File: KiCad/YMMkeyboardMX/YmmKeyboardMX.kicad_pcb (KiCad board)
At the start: 2 copper layers, 259.1 x 139.7 mm, 123 parts, among them J3 RGB, SW10 SW_Push, SW11 SW_Push, SW12 SW_Push, SW13 SW_Push, SW14 SW_Push, SW15 SW_Push, SW16 SW_Push, SW17 SW_Push, SW18 SW_Push, SW19 SW_Push, SW2 SW_Push, SW20 SW_Push, SW21 SW_Push, SW22 SW_Push, SW23 SW_Push, SW24 SW_Push, SW25 SW_Push, SW26 SW_Push, SW27 SW_Push, SW28 SW_Push, SW29 SW_Push, SW3 SW_Push, SW30 SW_Push, SW31 SW_Push, SW32 RotaryEncoder_Switch, SW4 SW_Push, SW5 SW_Push, SW6 SW_Push, SW7 SW_Push, SW8 SW_Push, SW9 SW_Push, U1 RP2040-Zero

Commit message: 3号機のcadデータ
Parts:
- removed J3: RGB, Connector_PinSocket_2.54mm:PinSocket_1x03_P2.54mm_Vertical
- added D1: SK6812, LED_SMD:LED_SK6812_PLCC4_5.0x5.0mm_P3.2mm, F.Cu at (135.9, 40.6)
- C1, C10, C11, C12, C13, C14, C15, C16, C17, C18, C19, C2, C20, C21, C22, C23, C24, C25, C26, C27, C28, C29, C3, C30, C4, C5, C6, C7, C8, C9: moved to B.Cu
- D10, D11, D12, D13, D14, D15, D16, D17, D18, D19, D2, D20, D21, D22, D23, D24, D25, D26, D27, D28, D29, D3, D30, D31, D32, D4, D5, D6, D7, D8, D9: moved to F.Cu
- SW10, SW11, SW12, SW13, SW14, SW15, SW16, SW17, SW18, SW19, SW2, SW20, SW21, SW22, SW23, SW24, SW25, SW26, SW27, SW28, SW29, SW3, SW30, SW31, SW4, SW5, SW6, SW7, SW8, SW9: footprint isw-kbd:CherryMX_Hotswap_1u -> Button_Switch_THT:SW_PUSH_6mm
- moved D37 208.6 mm to (199.5, 40.3)
- moved D36 194.4 mm to (186.8, 40.3)
- moved D43 192.1 mm to (199.5, 58.1)
- moved D35 181.3 mm to (175.3, 40.3)
- moved D42 178.9 mm to (188.1, 58.1)
- moved D49 175.0 mm to (199.5, 78.4)
- moved D34 167.1 mm to (162.7, 40.3)
- moved D32 164.8 mm to (224.8, 53.3), turned to 90 degrees
- moved D41 164.6 mm to (175.3, 58.1)
- moved C6 163.0 mm to (199.8, 40.6), turned to 180 degrees
- moved D48 160.7 mm to (186.8, 78.4)
- moved D55 160.3 mm to (200.8, 98.7)
- moved C12 158.4 mm to (204.5, 58.4), turned to 180 degrees
- moved C24 155.0 mm to (207.0, 97.8), turned to 180 degrees
- moved C18 153.6 mm to (205.7, 77.5), turned to 180 degrees
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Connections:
- net Net-(D1-VDD) renamed +5V
- U1 pad 9: Net-(J3-Pin_3) -> unconnected-(U1-Pad9)
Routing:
- net Net-(D1-DIN): track 0.00 -> 139.3 mm, vias 0 -> 1
- net Net-(D37-DOUT): track 0.00 -> 94.0 mm, vias 0 -> 2
- net Net-(SW32-PadS1): track 0.00 -> 93.2 mm, vias 0 -> 2
- net Net-(SW14-Pad1): track 97.5 -> 189.7 mm, vias 0 -> 1
- net Net-(SW32-PadA): track 0.00 -> 91.4 mm
- net Net-(D49-DOUT): track 0.00 -> 90.0 mm, vias 0 -> 2
- net Net-(D43-DOUT): track 0.00 -> 82.4 mm, vias 0 -> 2
- net Net-(SW32-PadB): track 0.00 -> 81.9 mm
- net Net-(D55-DOUT): track 0.00 -> 80.3 mm, vias 0 -> 2
- net Net-(SW15-Pad1): track 97.5 -> 175.8 mm, vias 0 -> 2
- net Net-(D14-K): track 40.8 -> 117.0 mm
- net Net-(SW10-Pad1): track 97.5 -> 169.0 mm
- net Net-(D32-K): track 0.00 -> 63.3 mm
- net Net-(SW11-Pad1): track 97.5 -> 149.6 mm
- net Net-(D2-K): track 116.5 -> 155.9 mm
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- added copper zone on In2.Cu, net +5V
- added copper zone on In1.Cu, net GND
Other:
- board size 259.1 x 139.7 mm -> 99.9 x 99.7 mm
- copper layers 2 -> 4
- board text added: "K"
- board text added: "USB"

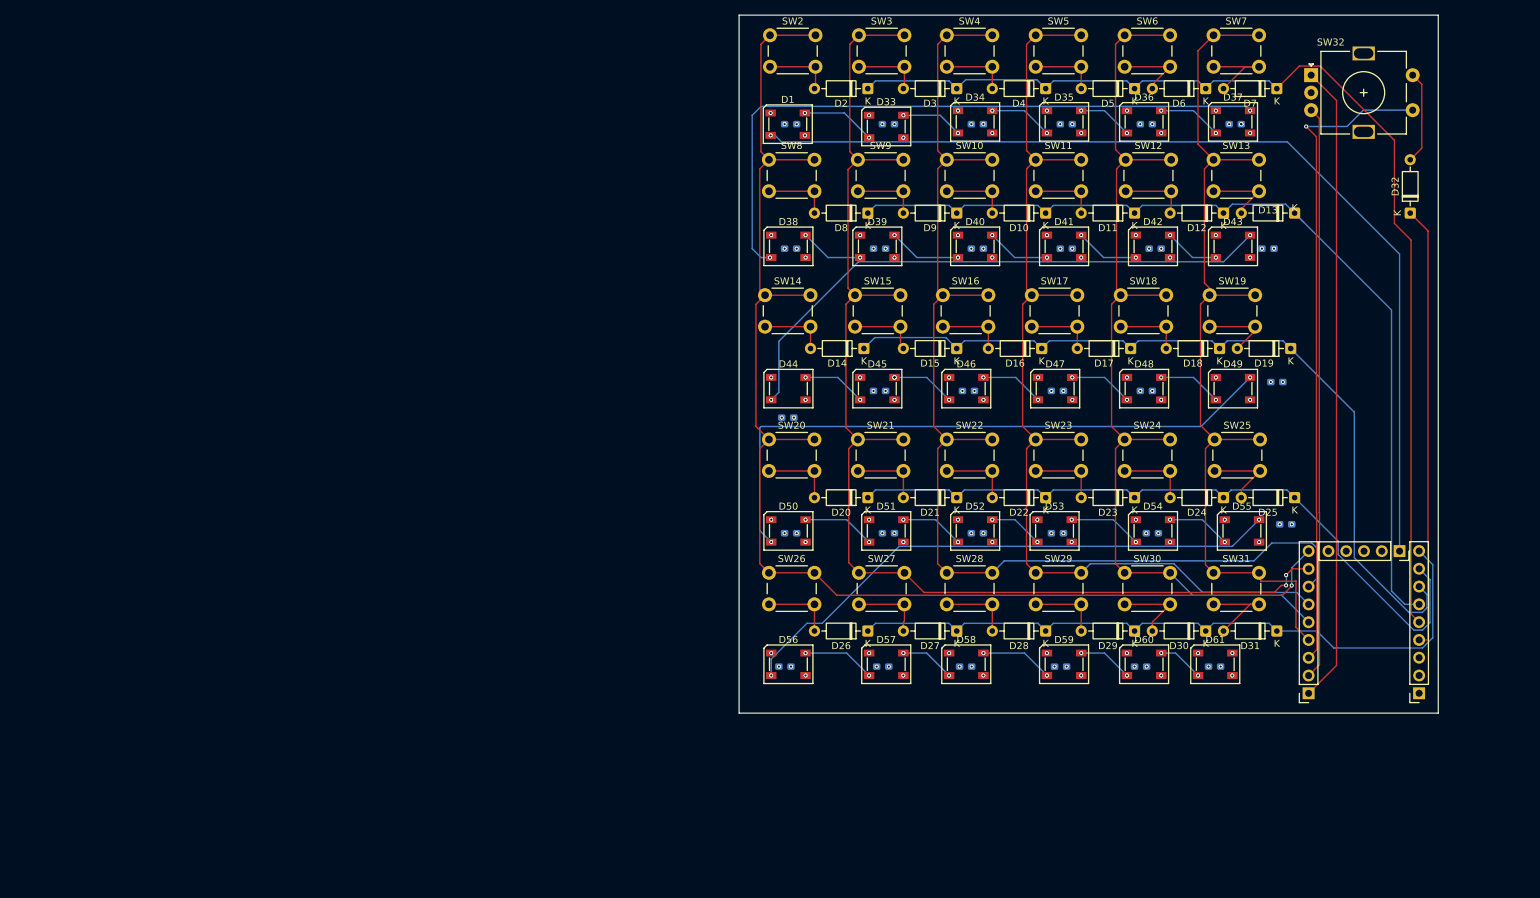
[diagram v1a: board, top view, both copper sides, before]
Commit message: 3号機発注
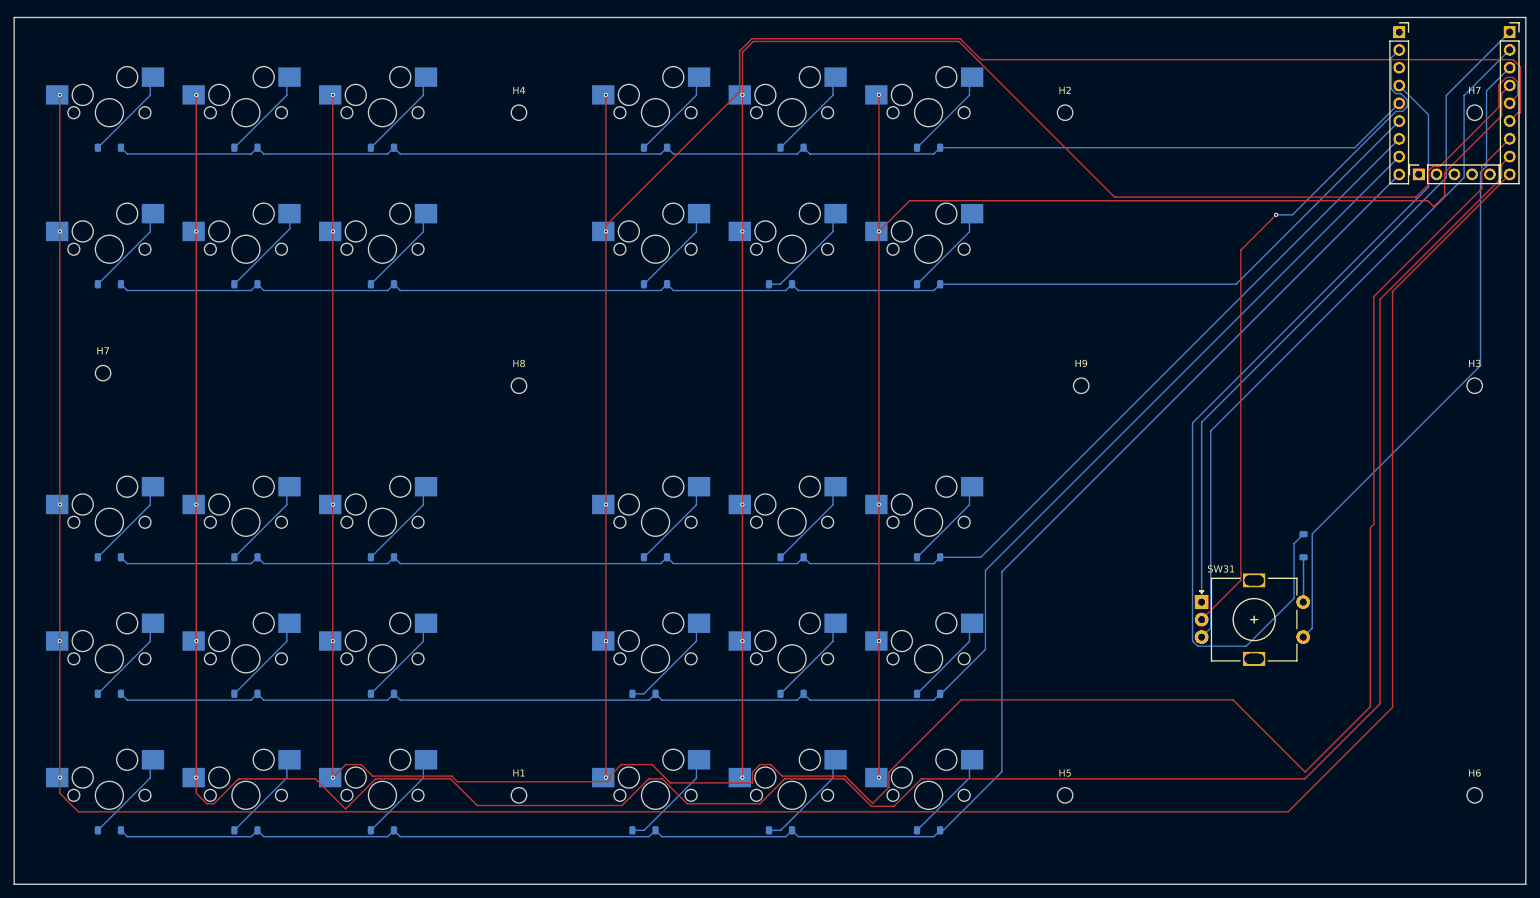
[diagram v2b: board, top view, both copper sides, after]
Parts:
- removed C1, C10, C11, C12, C13, C14, C15, C16, C17, C18, C19, C2, C20, C21, C22, C23, C24, C25, C26, C27, C28, C29, C3, C30, C4, C5, C6, C7, C8, C9: 0.1uF, Capacitor_SMD:C_0603_1608Metric_Pad1.08x0.95mm_HandSolder
- removed D32: 1N4148, Diode_THT:D_DO-35_SOD27_P7.62mm_Horizontal
- removed D33, D34, D35, D36, D37, D38, D39, D40, D41, D42, D43, D44, D45, D46, D47, D48, D49, D50, D51, D52, D53, D54, D55, D56, D57, D58, D59, D60, D61: SK6812, LED_SMD:LED_SK6812_PLCC4_5.0x5.0mm_P3.2mm
- removed SW32: RotaryEncoder_Switch, Rotary_Encoder:RotaryEncoder_Alps_EC11E-Switch_Vertical_H20mm
- added H1: MountingHole, MountingHole:MountingHole_2.2mm_M2, F.Cu at (97.5, 136.5)
- added H2: MountingHole, MountingHole:MountingHole_2.2mm_M2, F.Cu at (175.5, 39.0)
- added H3: MountingHole, MountingHole:MountingHole_2.2mm_M2, F.Cu at (234.0, 78.0)
- added H4: MountingHole, MountingHole:MountingHole_2.2mm_M2, F.Cu at (97.5, 39.0)
- added H5: MountingHole, MountingHole:MountingHole_2.2mm_M2, F.Cu at (175.5, 136.5)
- added H6: MountingHole, MountingHole:MountingHole_2.2mm_M2, F.Cu at (234.0, 136.5)
- added H7: MountingHole, MountingHole:MountingHole_2.2mm_M2, F.Cu at (38.1, 76.2)
- added H7: MountingHole, MountingHole:MountingHole_2.2mm_M2, F.Cu at (234.0, 39.0)
- added H8: MountingHole, MountingHole:MountingHole_2.2mm_M2, F.Cu at (97.5, 78.0)
- added H9: MountingHole, MountingHole:MountingHole_2.2mm_M2, F.Cu at (177.8, 78.0)
- added SW1: SW_Push, isw-kbd:CherryMX_Hotswap_1u, F.Cu at (39.0, 39.0)
- D1: value SK6812 -> 1N4148; footprint LED_SMD:LED_SK6812_PLCC4_5.0x5.0mm_P3.2mm -> Diode_SMD:D_SOD-123; moved to B.Cu
- D10, D11, D12, D13, D14, D15, D16, D17, D18, D19, D2, D20, D21, D22, D23, D24, D25, D26, D27, D28, D29, D3, D30, D31, D4, D5, D6, D7, D8, D9: footprint Diode_THT:D_DO-35_SOD27_P7.62mm_Horizontal -> Diode_SMD:D_SOD-123; moved to B.Cu
- SW10, SW11, SW12, SW13, SW14, SW15, SW16, SW17, SW18, SW19, SW2, SW20, SW21, SW22, SW23, SW24, SW25, SW26, SW27, SW28, SW29, SW3, SW30, SW4, SW5, SW6, SW7, SW8, SW9: footprint Button_Switch_THT:SW_PUSH_6mm -> isw-kbd:CherryMX_Hotswap_1u
- SW31: value SW_Push -> RotaryEncoder_Switch; footprint Button_Switch_THT:SW_PUSH_6mm -> Rotary_Encoder:RotaryEncoder_Alps_EC11E-Switch_Vertical_H20mm
- moved D13 176.3 mm to (39.0, 102.5)
- moved D25 175.8 mm to (39.0, 141.5)
- moved D19 175.8 mm to (39.0, 122.0)
- moved D7 169.1 mm to (39.0, 63.5)
- moved SW13 166.0 mm to (39.0, 97.5)
- moved SW25 165.8 mm to (39.0, 136.5)
- moved SW19 165.5 mm to (39.0, 117.0)
- moved SW7 160.6 mm to (39.0, 58.5)
- moved D1 96.9 mm to (39.0, 44.0), turned to 180 degrees
- moved D26 93.3 mm to (58.5, 141.5)
- moved D14 93.2 mm to (58.5, 102.5)
- moved D20 93.1 mm to (58.5, 122.0)
- moved D8 89.4 mm to (58.5, 63.5)
- moved D2 89.2 mm to (58.5, 44.0)
- moved D15 87.3 mm to (78.0, 102.5)
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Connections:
- D1 pad 1: GND -> Net-(D1-K)
- D1 pad 2: Net-(D1-DIN) -> Net-(D1-A)
- D13 pad 1: Net-(D10-K) -> Net-(D13-K)
- D14 pad 1: Net-(D14-K) -> Net-(D13-K)
- D15 pad 1: Net-(D14-K) -> Net-(D13-K)
- D16 pad 1: Net-(D14-K) -> Net-(D13-K)
- D17 pad 1: Net-(D14-K) -> Net-(D13-K)
- D18 pad 1: Net-(D14-K) -> Net-(D13-K)
- D19 pad 1: Net-(D14-K) -> Net-(D19-K)
- D2 pad 1: Net-(D2-K) -> Net-(D1-K)
- D20 pad 1: Net-(D20-K) -> Net-(D19-K)
- D21 pad 1: Net-(D20-K) -> Net-(D19-K)
- D22 pad 1: Net-(D20-K) -> Net-(D19-K)
- D23 pad 1: Net-(D20-K) -> Net-(D19-K)
- D24 pad 1: Net-(D20-K) -> Net-(D19-K)
- D25 pad 1: Net-(D20-K) -> Net-(D25-K)
- D26 pad 1: Net-(D26-K) -> Net-(D25-K)
- D27 pad 1: Net-(D26-K) -> Net-(D25-K)
- D28 pad 1: Net-(D26-K) -> Net-(D25-K)
- D29 pad 1: Net-(D26-K) -> Net-(D25-K)
- D3 pad 1: Net-(D2-K) -> Net-(D1-K)
- D30 pad 1: Net-(D26-K) -> Net-(D25-K)
- D31 pad 1: Net-(D26-K) -> Net-(D31-K)
- D4 pad 1: Net-(D2-K) -> Net-(D1-K)
- D5 pad 1: Net-(D2-K) -> Net-(D1-K)
- D6 pad 1: Net-(D2-K) -> Net-(D1-K)
- D7 pad 1: Net-(D2-K) -> Net-(D10-K)
- SW13 pad 1: Net-(SW13-Pad1) -> Net-(SW1-Pad1)
- SW19 pad 1: Net-(SW13-Pad1) -> Net-(SW1-Pad1)
- SW25 pad 1: Net-(SW13-Pad1) -> Net-(SW1-Pad1)
- SW7 pad 1: Net-(SW13-Pad1) -> Net-(SW1-Pad1)
- U1 pad 0: Net-(SW32-PadA) -> Net-(SW31-PadA)
- U1 pad 1: Net-(SW32-PadB) -> Net-(SW31-PadB)
- U1 pad 13: Net-(D1-DIN) -> unconnected-(U1-Pad13)
- U1 pad 14: Net-(D26-K) -> Net-(D25-K)
- U1 pad 15: Net-(D20-K) -> Net-(D19-K)
- U1 pad 2: Net-(SW32-PadS1) -> Net-(SW31-PadS1)
- U1 pad 26: Net-(D14-K) -> Net-(D13-K)
- U1 pad 28: Net-(D2-K) -> Net-(D1-K)
- U1 pad 29: Net-(D32-K) -> Net-(D31-K)
- U1 pad 3: Net-(SW13-Pad1) -> Net-(SW12-Pad1)
- U1 pad 30: unconnected-(U1-3V3-Pad30) -> +3.3V
- U1 pad 4: Net-(SW12-Pad1) -> Net-(SW11-Pad1)
- U1 pad 5: Net-(SW11-Pad1) -> Net-(SW10-Pad1)
- U1 pad 6: Net-(SW10-Pad1) -> Net-(SW15-Pad1)
- U1 pad 7: Net-(SW15-Pad1) -> Net-(SW14-Pad1)
- U1 pad 8: Net-(SW14-Pad1) -> Net-(SW1-Pad1)
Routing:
- net Net-(SW1-Pad1): track 0.00 -> 380.4 mm, vias 0 -> 5
- net Net-(D25-K): track 0.00 -> 241.8 mm
- net Net-(D19-K): track 0.00 -> 224.7 mm
- net Net-(D13-K): track 0.00 -> 211.1 mm
- net Net-(D1-K): track 0.00 -> 188.9 mm
- net Net-(SW14-Pad1): track 189.7 -> 374.1 mm, vias 1 -> 5
- net Net-(SW15-Pad1): track 175.8 -> 359.0 mm, vias 2 -> 5
- net Net-(D2-K): track 155.9 -> 0.00 mm
- net Net-(D1-DIN): track 139.3 -> 0.00 mm, vias 1 -> 0
- net Net-(SW13-Pad1): track 130.7 -> 0.00 mm
- net Net-(D31-K): track 0.00 -> 122.4 mm
- net Net-(D14-K): track 117.0 -> 0.00 mm
- net Net-(D20-K): track 102.6 -> 0.00 mm
- net Net-(SW31-PadB): track 0.00 -> 102.1 mm
- net Net-(D26-K): track 100.1 -> 0.00 mm
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- removed copper zone on In2.Cu, net +5V
- removed copper zone on In1.Cu, net GND
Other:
- board size 99.9 x 99.7 mm -> 215.9 x 123.8 mm
- copper layers 4 -> 2
- board text removed: "K"
- board text removed: "USB"
